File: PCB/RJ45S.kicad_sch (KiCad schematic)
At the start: 2 parts

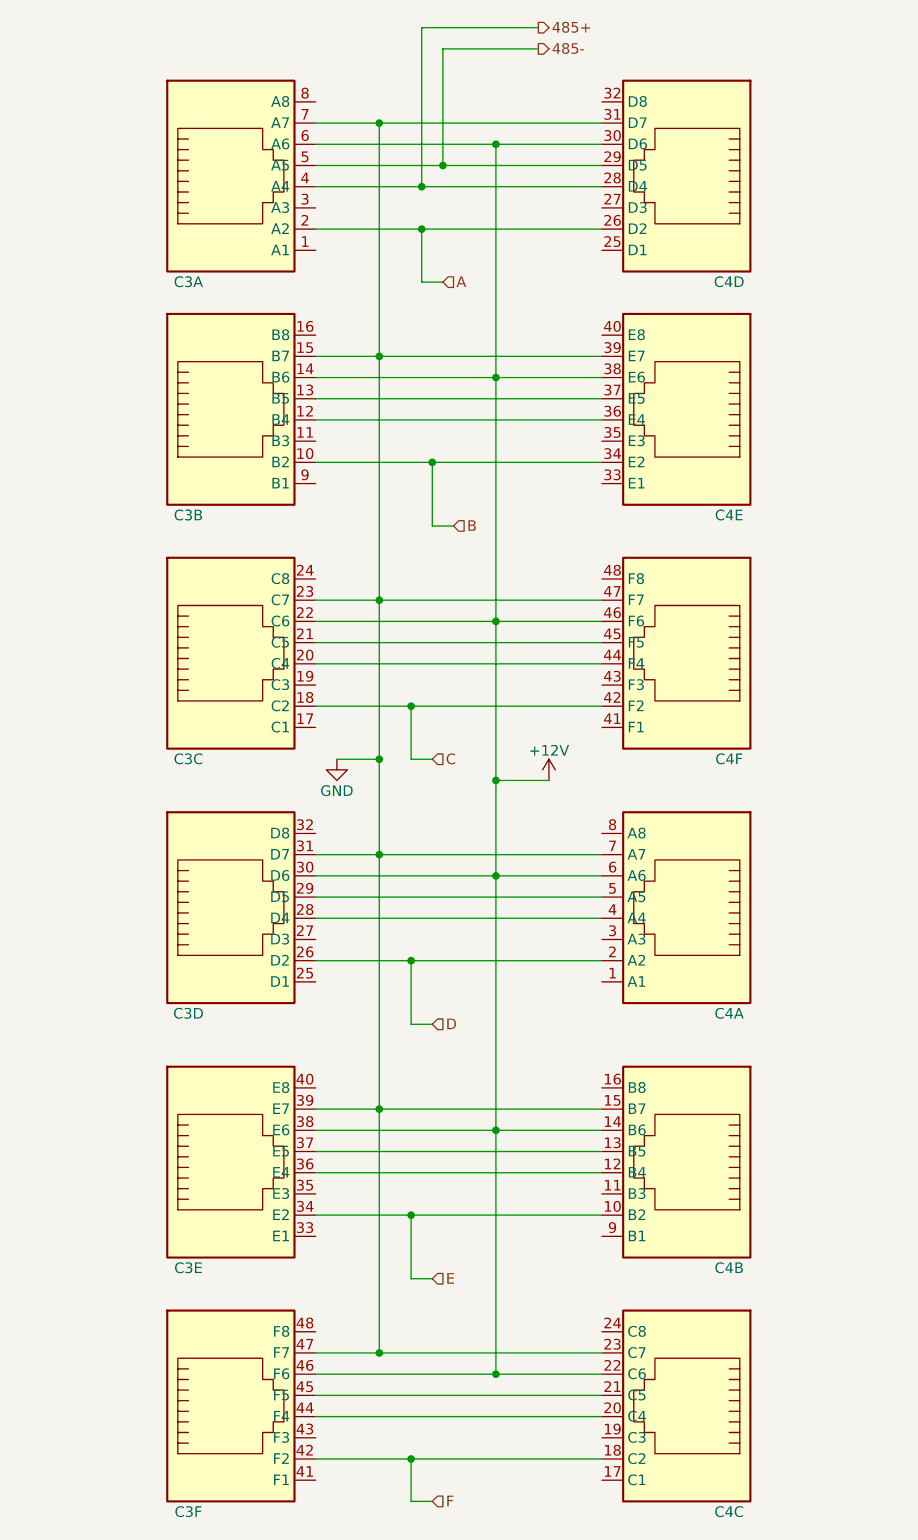
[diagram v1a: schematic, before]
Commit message: Version 2 of PCB
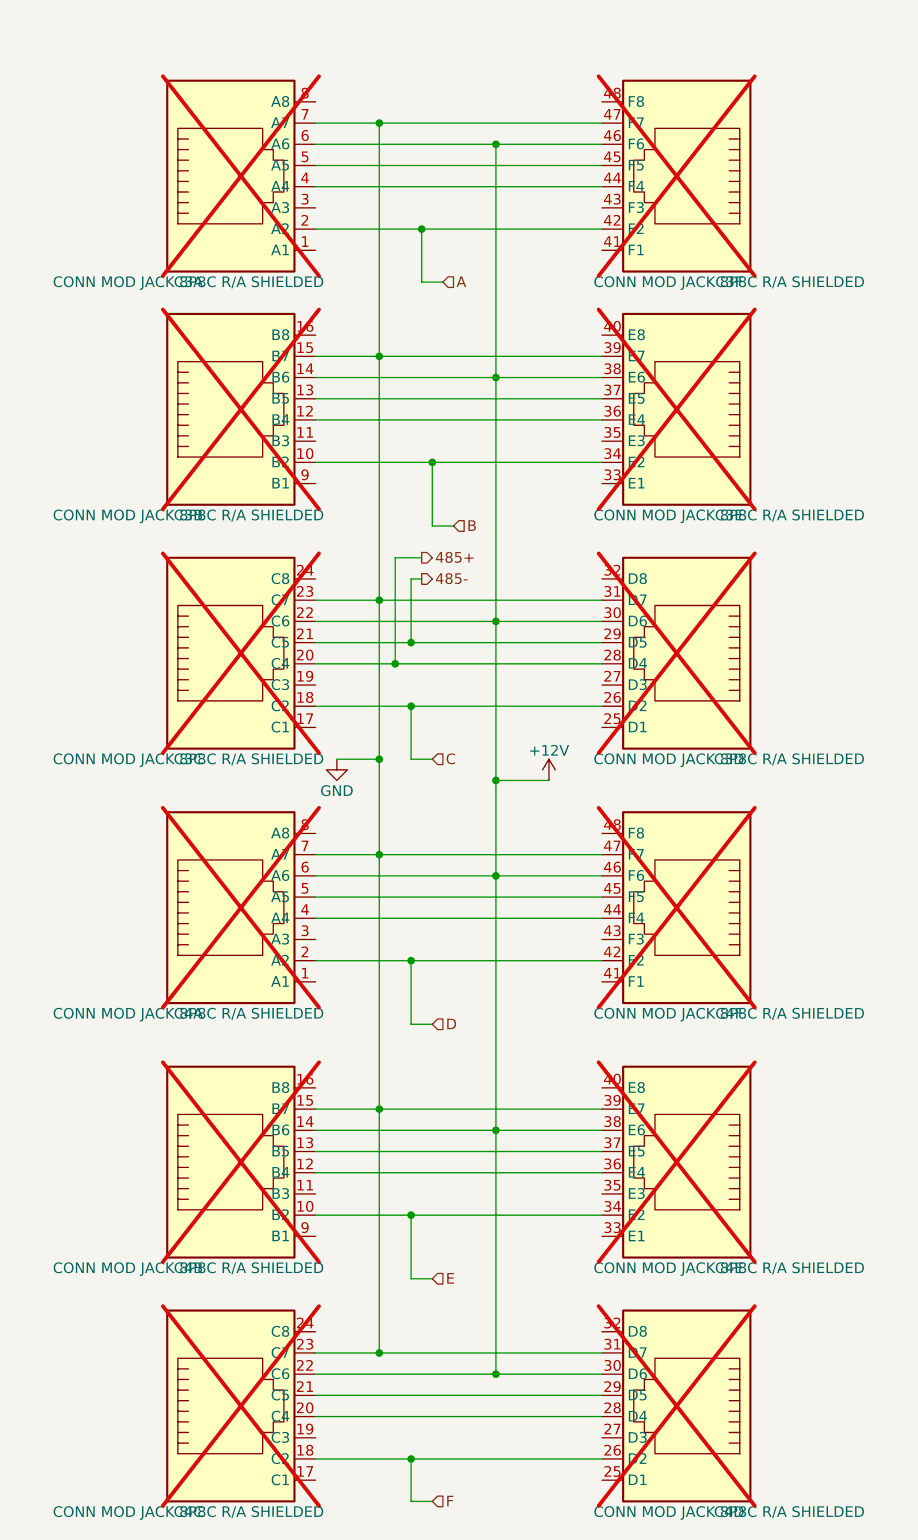
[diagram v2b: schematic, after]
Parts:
- C3, C4: value ~ -> CONN MOD JACK 8P8C R/A SHIELDED; now not fitted
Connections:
- net +12V: now also C4.14 (B6), C4.22 (C6), C4.30 (D6), C4.38 (E6), C4.46 (F6), C4.6 (A6); no longer C4.14 (B6), C4.22 (C6), C4.30 (D6), C4.38 (E6), C4.46 (F6), C4.6 (A6)
- net 485+: now also C3.20 (C4), C3.28 (D4); no longer C3.4 (A4), C4.28 (D4)
- net 485-: now also C3.21 (C5), C3.29 (D5); no longer C3.5 (A5), C4.29 (D5)
- net A: now also C3.42 (F2); no longer C4.26 (D2)
- net B: now also C3.34 (E2); no longer C4.34 (E2)
- net C: now also C3.26 (D2); no longer C4.42 (F2)
- net D: now also C4.2 (A2), C4.42 (F2); no longer C3.26 (D2), C4.2 (A2)
- net E: now also C4.10 (B2), C4.34 (E2); no longer C3.34 (E2), C4.10 (B2)
- net F: now also C4.18 (C2), C4.26 (D2); no longer C3.42 (F2), C4.18 (C2)
- net GND: now also C4.15 (B7), C4.23 (C7), C4.31 (D7), C4.39 (E7), C4.47 (F7), C4.7 (A7); no longer C4.15 (B7), C4.23 (C7), C4.31 (D7), C4.39 (E7), C4.47 (F7), C4.7 (A7)
- net at C3.44 (F4): now also C3.4 (A4); no longer C4.20 (C4)
- net at C3.45 (F5): now also C3.5 (A5); no longer C4.21 (C5)
- net at C3.12 (B4): now also C3.36 (E4); no longer C4.36 (E4)
- net at C3.13 (B5): now also C3.37 (E5); no longer C4.37 (E5)
- new net: C4.4 (A4), C4.44 (F4)
- new net: C4.45 (F5), C4.5 (A5)
- new net: C4.20 (C4), C4.28 (D4)
- new net: C4.21 (C5), C4.29 (D5)
- new net: C4.12 (B4), C4.36 (E4)
- new net: C4.13 (B5), C4.37 (E5)
